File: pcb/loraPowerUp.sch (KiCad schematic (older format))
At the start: 10 parts, among them P1_L1 IN_LEFT, P1_R1 IN_RIGHT, P2_L1 DORGI_L, P2_R1 DORGI_R, P3 LORA, Q1 Q_NPN_BCE, Q2 IRF9540N

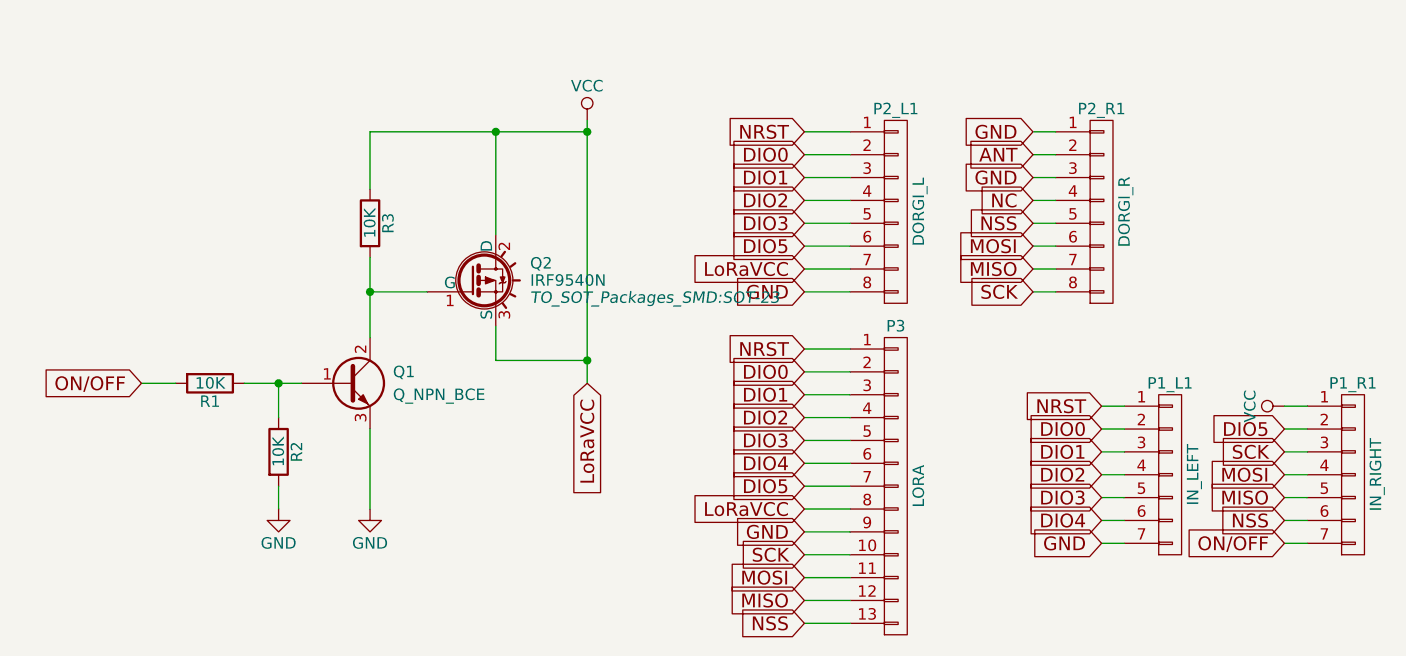
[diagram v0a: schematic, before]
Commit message: Fixing VCC
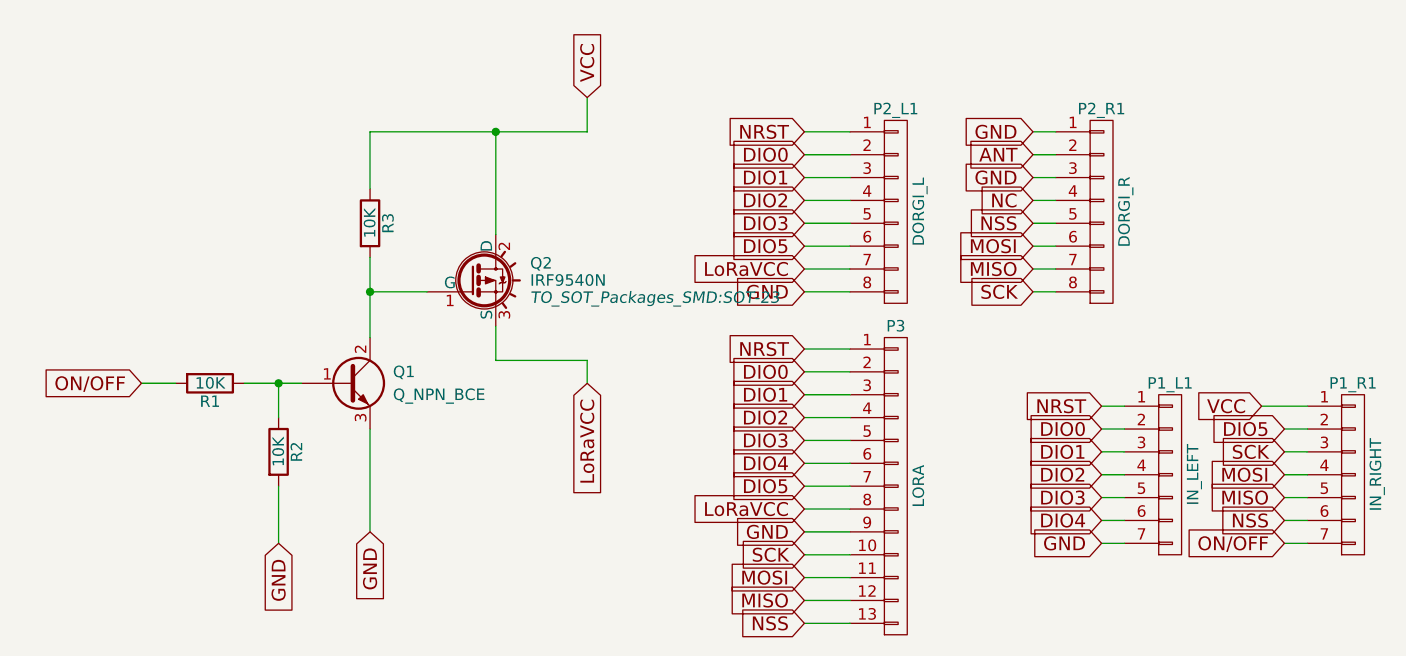
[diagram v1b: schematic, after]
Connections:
- net VCC: no longer P2_L1.7 (P7), P3.8 (P8), Q2.3 (S)
- new net LoRaVCC: P2_L1.7 (P7), P3.8 (P8), Q2.3 (S)
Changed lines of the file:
@@
 	3150 2150 3150 2000
 Connection ~ 3150 2000
-$Comp
-L GND #PWR01
-U 1 1 5AE44DA6
-P 3150 2550
-F 0 "#PWR01" H 3150 2300 50  0001 C CNN
-F 1 "GND" H 3150 2400 50  0000 C CNN
-F 2 "" H 3150 2550 50  0000 C CNN
-F 3 "" H 3150 2550 50  0000 C CNN
-	1    3150 2550
-	1    0    0    -1
-$EndComp
 Wire Wire Line
-	3150 2550 3150 2450
-$Comp
-L GND #PWR02
-U 1 1 5AE44FD3
-P 3550 2550
-F 0 "#PWR02" H 3550 2300 50  0001 C CNN
-F 1 "GND" H 3550 2400 50  0000 C CNN
-F 2 "" H 3550 2550 50  0000 C CNN
-F 3 "" H 3550 2550 50  0000 C CNN
-	1    3550 2550
-	1    0    0    -1
-$EndComp
+	3150 2450 3150 2700
 Wire Wire Line
 	3550 1450 3550 1800
@@
 	3550 1600 3800 1600
 Connection ~ 3550 1600
-$Comp
-L VCC #PWR03
-U 1 1 5AE4543B
-P 4500 850
-F 0 "#PWR03" H 4500 700 50  0001 C CNN
-F 1 "VCC" H 4500 1000 50  0000 C CNN
-F 2 "" H 4500 850 50  0000 C CNN
-F 3 "" H 4500 850 50  0000 C CNN
-	1    4500 850
-	1    0    0    -1
-$EndComp
 Wire Wire Line
 	3550 1150 3550 900
-Wire Wire Line
-	3550 900  4500 900
 Text GLabel 4500 2000 3    60   Input ~ 0
 LoRaVCC
@@
 Text GLabel 7550 2200 0    60   Input ~ 0
 DIO5
-$Comp
-L VCC #PWR04
-U 1 1 5AE47F33
-P 7550 2100
-F 0 "#PWR04" H 7550 1950 50  0001 C CNN
-F 1 "VCC" H 7550 2250 50  0000 C CNN
-F 2 "" H 7550 2100 50  0000 C CNN
-F 3 "" H 7550 2100 50  0000 C CNN
-	1    7550 2100
-	0    -1   -1   0
-$EndComp
 Text GLabel 6750 2700 0    60   Input ~ 0
 GND
@@
 	6750 2700 6850 2700
 Wire Wire Line
-	7550 2100 7650 2100
+	7450 2100 7650 2100
 Connection ~ 4100 900
 Wire Wire Line
-	4500 850  4500 2000
-Wire Wire Line
 	4100 900  4100 1350
-Connection ~ 4500 900
 Wire Wire Line
 	4100 1750 4100 1900
 Wire Wire Line
-	4100 1900 4500 1900
-Connection ~ 4500 1900
-Wire Wire Line
 	2550 2000 2700 2000
 Wire Wire Line
-	3550 2550 3550 2200
+	3550 2200 3550 2650
+Wire Wire Line
+	4500 1900 4500 2000
+Wire Wire Line
+	4100 1900 4500 1900
+Wire Wire Line
+	3550 900  4500 900
+Wire Wire Line
+	4500 900  4500 750
+Text GLabel 4500 750  1    60   Input ~ 0
+VCC
+Text GLabel 3550 2650 3    60   Input ~ 0
+GND
+Text GLabel 7450 2100 0    60   Input ~ 0
+VCC
+Text GLabel 3150 2700 3    60   Input ~ 0
+GND
 $EndSCHEMATC
